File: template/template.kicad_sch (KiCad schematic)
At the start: 4 parts, among them SW1 MHPS2285

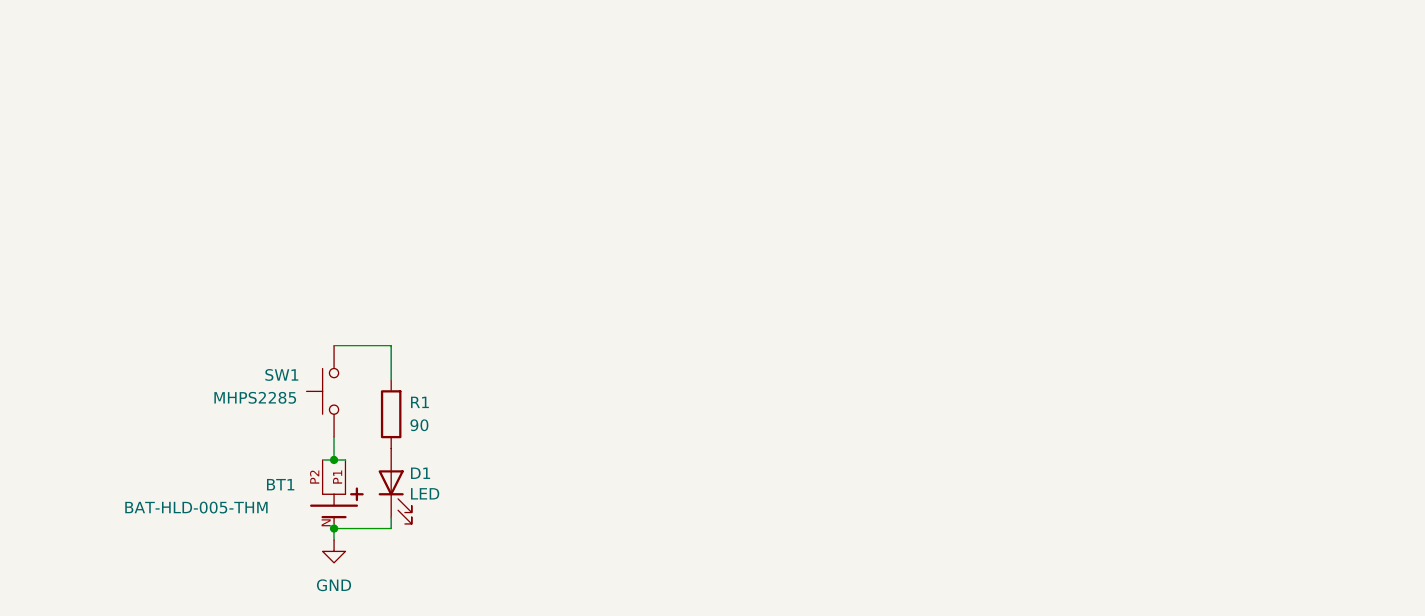
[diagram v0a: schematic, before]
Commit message: Template ready
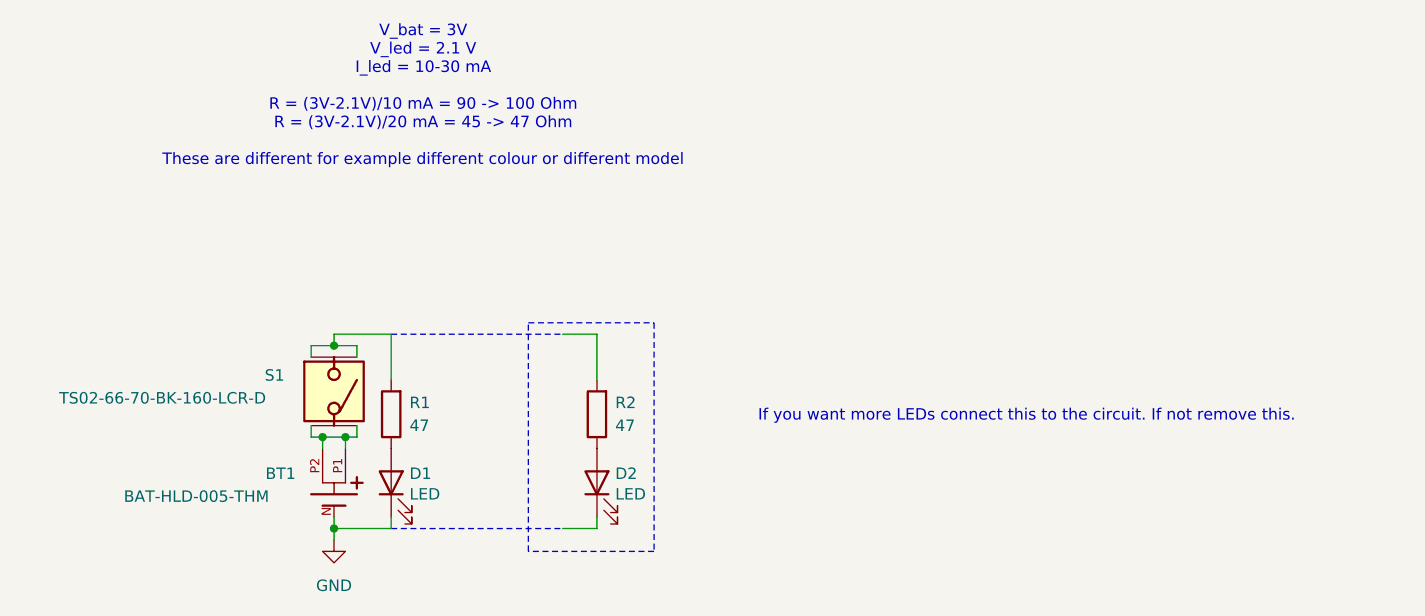
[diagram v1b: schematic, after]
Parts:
- removed SW1: MHPS2285, symbol Switch:SW_Push
- added D2: LED, LED_THT:LED_D5.0mm, symbol Device:LED
- added R2: 47, Resistor_THT:R_Axial_DIN0309_L9.0mm_D3.2mm_P15.24mm_Horizontal, symbol Device:R
- added S1: TS02-66-70-BK-160-LCR-D, Robot Uprising:SW_TS02-66-70-BK-160-LCR-D, symbol Robot Uprising:TS02-66-70-BK-160-LCR-D
- BT1: footprint -Robot Uprising:BAT-HLD-005-THM -> Robot Uprising:BAT-HLD-005-THM
- R1: value 90 -> 47; footprint (none) -> Resistor_THT:R_Axial_DIN0309_L9.0mm_D3.2mm_P15.24mm_Horizontal
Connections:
- net at BT1.P1, BT1.P2: now also S1.3, S1.4
- net at R1.2: now also S1.1, S1.2
- new net: D2.2 (A), R2.1
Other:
- note added: "If you want more LEDs connect this to the circuit. If not remove this."
- note added: "V_bat = 3V V_led = 2.1 V I_led = 10-30 mA R = (3V-2.1V)/10 mA = 90 -> 100 Ohm R = (3V-2.1V)/20 mA = 45 -> 47 Ohm These are different for example different colour or different model"
- moved on the sheet: BT1
